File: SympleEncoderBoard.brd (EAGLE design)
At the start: 50.8 x 50.8 mm, 31 parts, among them IC1 STM32F446RET6

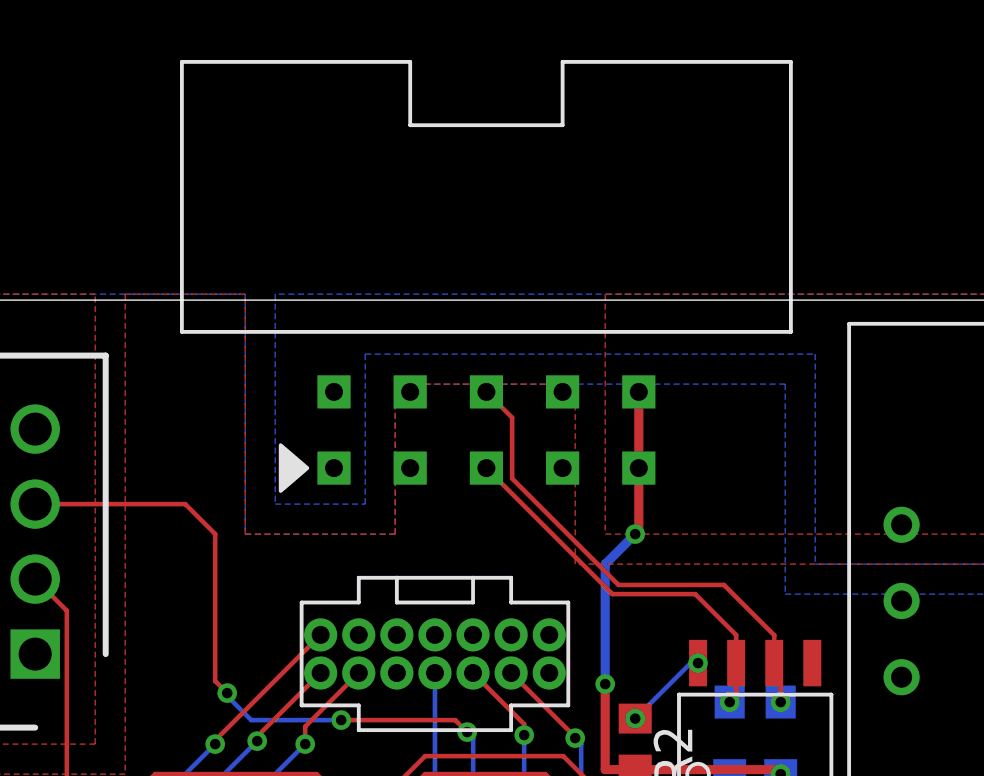
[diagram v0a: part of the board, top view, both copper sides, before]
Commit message: Add files via upload
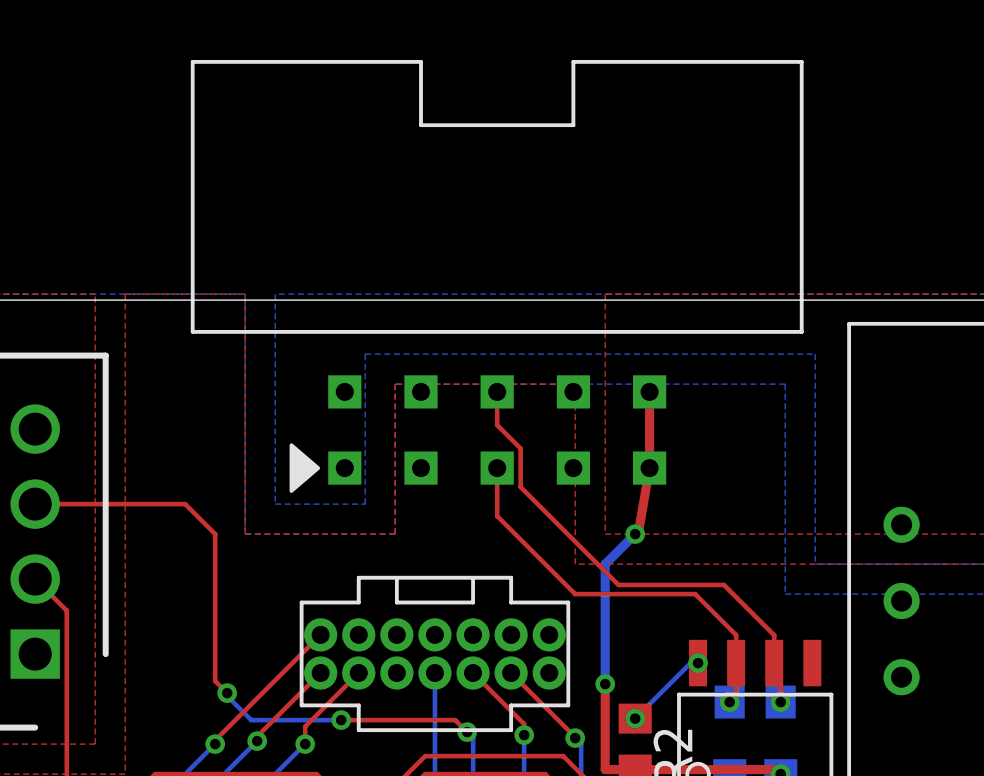
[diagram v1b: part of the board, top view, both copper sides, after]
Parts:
- moved BOX10P-L1 0.36 mm to (25.4, 47.7)
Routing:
- net CAN_H: track 13.0 -> 13.5 mm
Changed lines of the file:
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@@
 <attribute name="VALUE" x="37.04" y="17.625" size="1.27" layer="27"/>
 </element>
-<element name="BOX10P-L1" library="user_conector" package="BOX10P-L" value="BOX10PBOX10P-L" x="25.04" y="47.74" smashed="yes" rot="R180"/>
+<element name="BOX10P-L1" library="user_conector" package="BOX10P-L" value="BOX10PBOX10P-L" x="25.4" y="47.74" smashed="yes" rot="R180"/>
 <element name="C1" library="rcl" library_urn="urn:adsk.eagle:library:334" package="C1608" package3d_urn="urn:adsk.eagle:package:23621/2" value="1μ" x="18.69" y="25.23" smashed="yes" rot="MR270">
 <attribute name="NAME" x="17.055" y="25.865" size="1.27" layer="26" rot="MR270"/>
@@
 <via x="30" y="43" extent="1-16" drill="0.35"/>
 <wire x1="30" y1="43" x2="30.12" y2="43.12" width="0.3048" layer="1"/>
-<wire x1="30.12" y1="43.12" x2="30.12" y2="45.2" width="0.3048" layer="1"/>
-<wire x1="30.12" y1="45.2" x2="30.12" y2="47.74" width="0.3048" layer="1"/>
+<wire x1="30.12" y1="43.12" x2="30.48" y2="45.2" width="0.3048" layer="1"/>
+<wire x1="30.48" y1="45.2" x2="30.48" y2="47.74" width="0.3048" layer="1"/>
 <polygon width="0.1524" layer="1" thermals="no">
 <vertex x="29" y="51"/>
@@
 <wire x1="34.635" y1="38.7" x2="34.635" y2="39.6282875" width="0.1524" layer="1"/>
 <wire x1="34.635" y1="39.6282875" x2="32.9584875" y2="41.3048" width="0.1524" layer="1"/>
-<wire x1="25.8974" y1="46.8826" x2="25.04" y2="47.74" width="0.1524" layer="1"/>
-<wire x1="29.4439125" y1="41.3048" x2="25.8974" y2="44.8513125" width="0.1524" layer="1"/>
-<wire x1="25.8974" y1="44.8513125" x2="25.8974" y2="46.8826" width="0.1524" layer="1"/>
 <wire x1="32.9584875" y1="41.3048" x2="29.4439125" y2="41.3048" width="0.1524" layer="1"/>
+<wire x1="29.4439125" y1="41.3048" x2="26.1826" y2="44.5661125" width="0.1524" layer="1"/>
+<wire x1="26.1826" y1="44.5661125" x2="26.1826" y2="45.8486875" width="0.1524" layer="1"/>
+<wire x1="25.4" y1="46.6312875" x2="25.4" y2="47.74" width="0.1524" layer="1"/>
+<wire x1="26.1826" y1="45.8486875" x2="25.4" y2="46.6312875" width="0.1524" layer="1"/>
 </signal>
 <signal name="CAN_H">
@@
 <wire x1="32" y1="41" x2="33.365" y2="39.635" width="0.1524" layer="1"/>
 <wire x1="33.365" y1="39.635" x2="33.365" y2="38.7" width="0.1524" layer="1"/>
-<wire x1="32" y1="41" x2="29.24" y2="41" width="0.1524" layer="1"/>
-<wire x1="29.24" y1="41" x2="25.04" y2="45.2" width="0.1524" layer="1"/>
+<wire x1="25.4" y1="45.2" x2="25.4" y2="43.6" width="0.1524" layer="1"/>
+<wire x1="25.4" y1="43.6" x2="28" y2="41" width="0.1524" layer="1"/>
+<wire x1="28" y1="41" x2="32" y2="41" width="0.1524" layer="1"/>
 </signal>
 <signal name="+12V">
